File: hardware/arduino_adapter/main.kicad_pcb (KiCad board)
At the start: 2 copper layers, 60 x 66.5 mm, 15 parts, among them P1 CONN_8, P10 CONN_10, P11 CONN_8, P2 CONN_6, P3 CONN_6, P4 CONN_8, P5 POW, P6 TWI, P7 TWI_POW, P8 CONN_10, P9 CONN_8

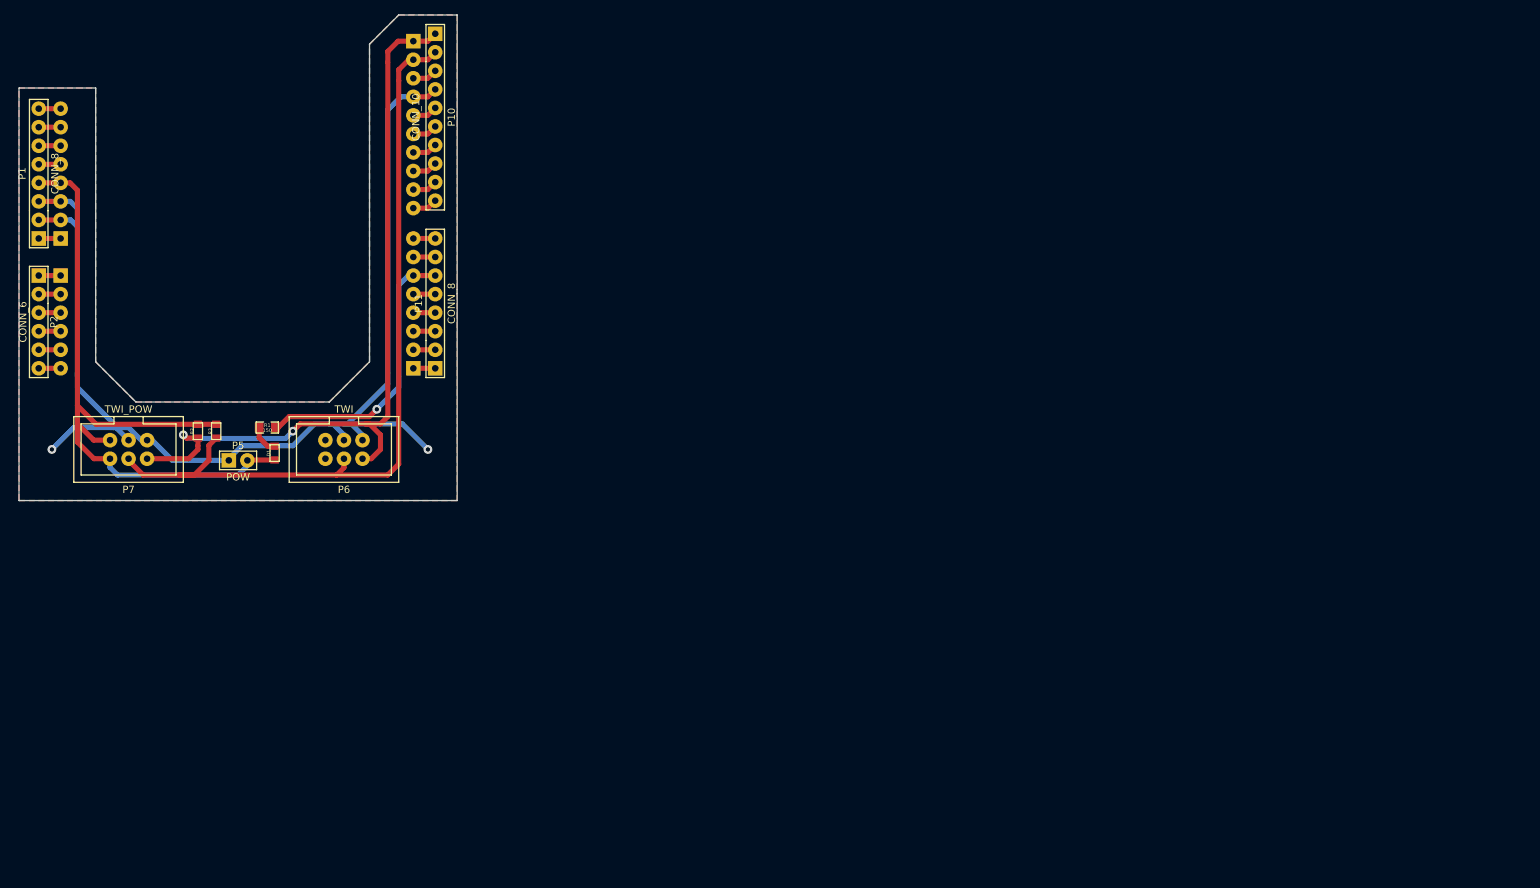
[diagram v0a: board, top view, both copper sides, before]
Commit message: order
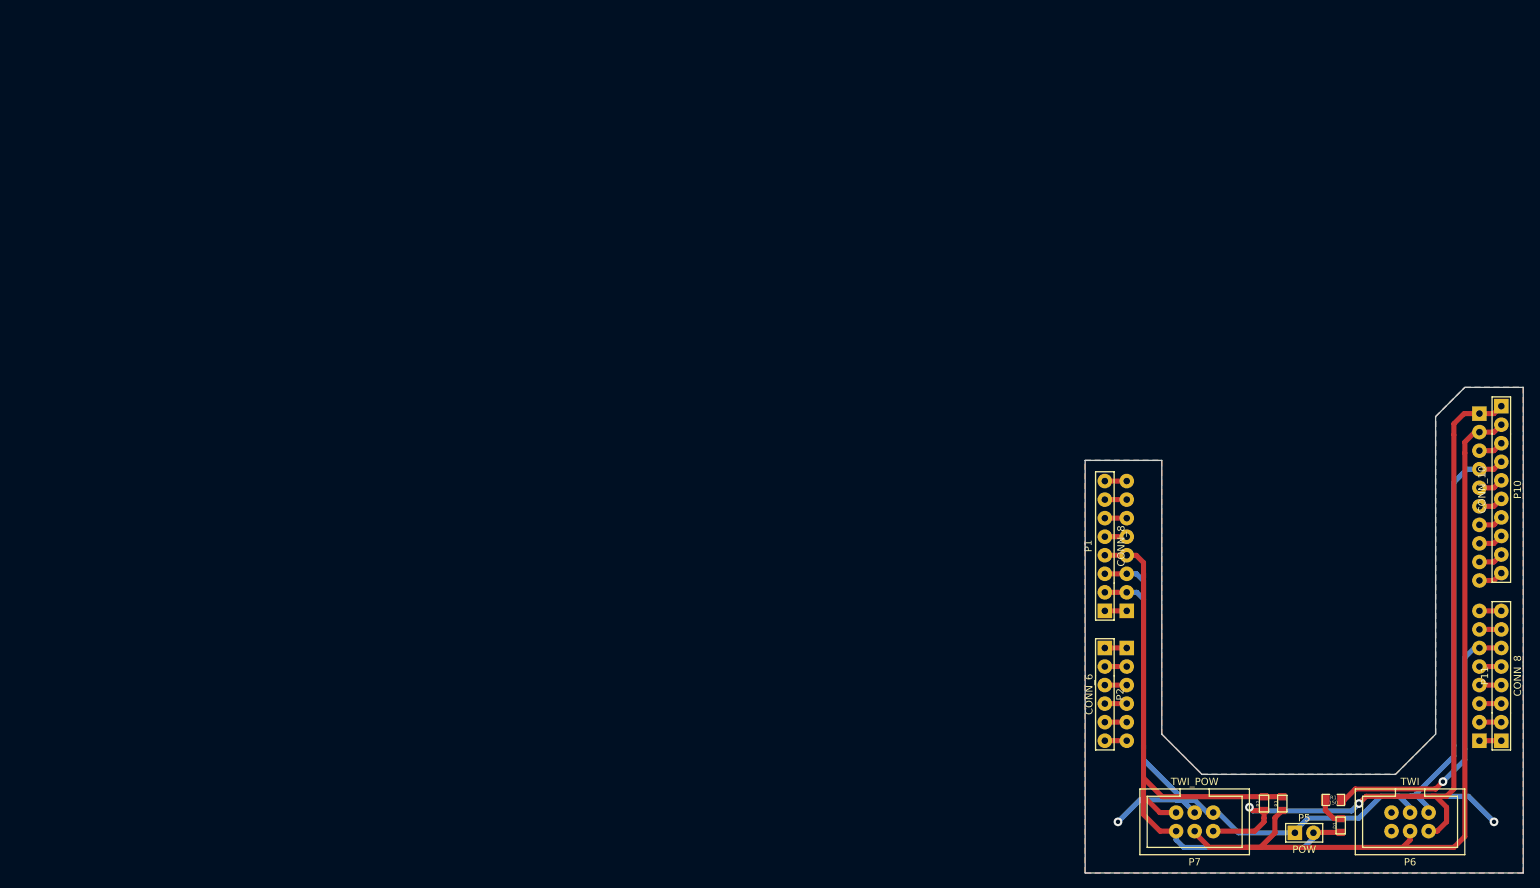
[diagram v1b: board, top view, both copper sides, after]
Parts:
- moved D1 154.7 mm to (241.0, 157.5)
- moved P1 154.7 mm to (208.7, 119.2)
- moved P10 154.7 mm to (263.0, 111.5)
- moved P11 154.7 mm to (263.0, 137.0)
- moved P2 154.7 mm to (208.7, 139.5)
- moved P3 154.7 mm to (211.7, 139.5)
- moved P4 154.7 mm to (211.7, 119.2)
- moved P5 154.7 mm to (236.0, 158.5)
- moved P6 154.7 mm to (250.5, 157.0)
- moved P7 154.7 mm to (221.0, 157.0)
- moved P8 154.7 mm to (260.0, 112.5)
- moved P9 154.7 mm to (260.0, 137.0)
- moved R1 154.7 mm to (240.0, 154.0)
- moved R2 154.7 mm to (230.5, 154.5)
- moved R3 154.7 mm to (233.0, 154.5)
